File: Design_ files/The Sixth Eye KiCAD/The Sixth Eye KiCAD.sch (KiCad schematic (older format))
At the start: 13 parts, among them J1 Battery conn, J2 US Sensor conn., J3 Vibration out, U1 ATmega328-AU, U2 LTC3525ISC6-5, Y1 8Mhz

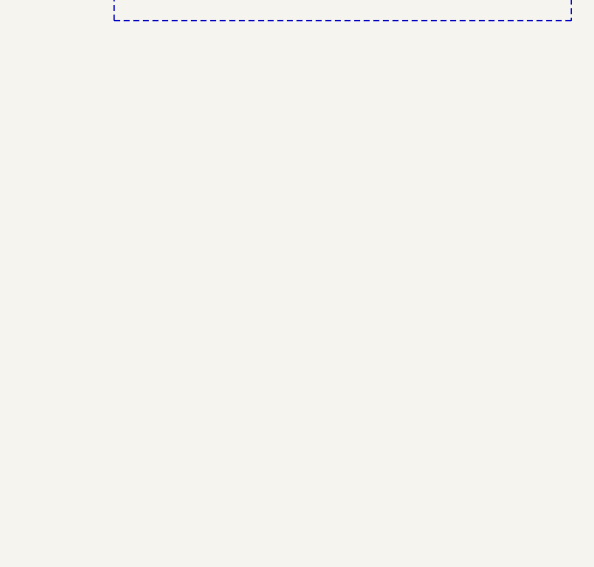
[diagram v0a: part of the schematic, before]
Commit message: ploted
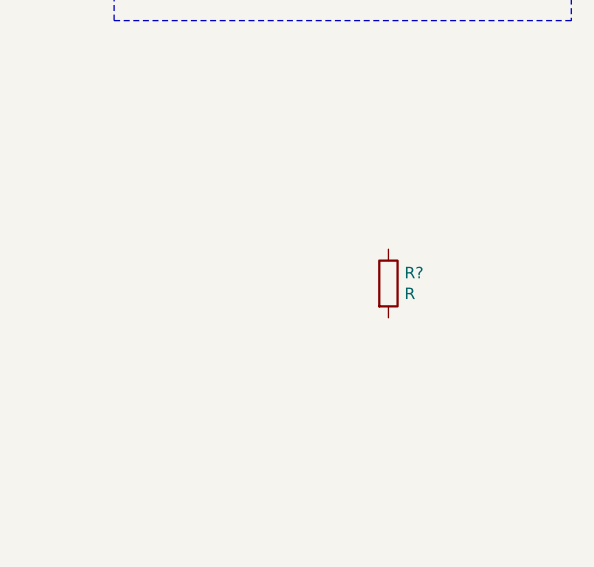
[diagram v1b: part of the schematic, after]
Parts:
- added R?: R, symbol Device:R
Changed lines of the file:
@@
 Wire Wire Line
 	4050 4850 4450 4850
+$Comp
+L Device:R R?
+U 1 1 6104FBF0
+P 8700 4950
+F 0 "R?" H 8770 4996 50  0000 L CNN
+F 1 "R" H 8770 4905 50  0000 L CNN
+F 2 "" V 8630 4950 50  0001 C CNN
+F 3 "~" H 8700 4950 50  0001 C CNN
+	1    8700 4950
+	1    0    0    -1
+$EndComp
 $EndSCHEMATC

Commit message: gerbers & drill files
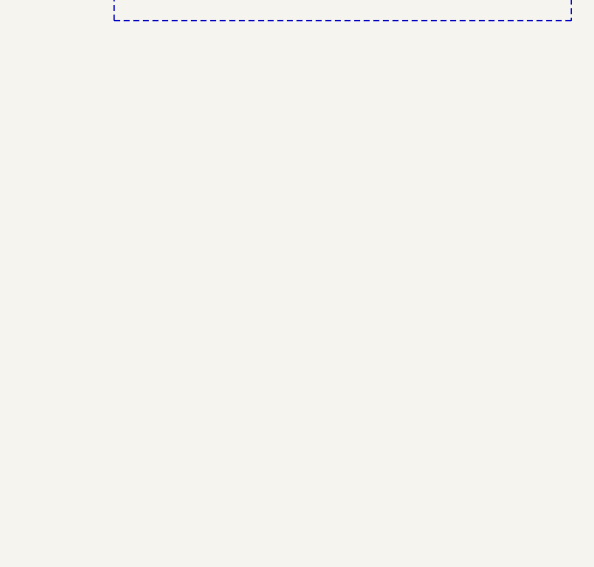
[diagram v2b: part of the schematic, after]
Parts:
- removed R?: R, symbol Device:R
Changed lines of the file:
@@
 Wire Wire Line
 	4050 4850 4450 4850
-$Comp
-L Device:R R?
-U 1 1 6104FBF0
-P 8700 4950
-F 0 "R?" H 8770 4996 50  0000 L CNN
-F 1 "R" H 8770 4905 50  0000 L CNN
-F 2 "" V 8630 4950 50  0001 C CNN
-F 3 "~" H 8700 4950 50  0001 C CNN
-	1    8700 4950
-	1    0    0    -1
-$EndComp
 $EndSCHEMATC
